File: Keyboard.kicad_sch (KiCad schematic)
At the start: 123 parts, among them SW1 MX_SW_solder, SW10 MX_SW_solder, SW11 MX_SW_solder, SW12 MX_SW_solder, SW13 MX_SW_solder, SW14 MX_SW_solder, SW15 MX_SW_solder, SW16 MX_SW_solder, SW17 MX_SW_solder, SW18 MX_SW_solder, SW19 MX_SW_solder, SW2 MX_SW_solder, SW20 MX_SW_solder, SW21 MX_SW_solder, SW22 MX_SW_solder, SW23 MX_SW_solder, SW24 MX_SW_solder, SW25 MX_SW_solder, SW26 MX_SW_solder, SW27 MX_SW_solder, SW28 MX_SW_solder, SW29 MX_SW_solder, SW3 MX_SW_solder, SW30 MX_SW_solder, SW31 MX_SW_solder, SW32 MX_SW_solder, SW33 MX_SW_solder, SW34 MX_SW_solder, SW35 MX_SW_solder, SW36 MX_SW_solder, SW37 MX_SW_solder, SW38 MX_SW_solder, SW39 MX_SW_solder, SW4 MX_SW_solder, SW40 MX_SW_solder, SW41 MX_SW_solder, SW42 MX_SW_solder, SW43 MX_SW_solder, SW44 MX_SW_solder, SW45 MX_SW_solder, SW46 MX_SW_solder, SW47 MX_SW_solder, SW48 MX_SW_solder, SW49 MX_SW_solder, SW5 MX_SW_solder, SW50 MX_SW_solder, SW51 MX_SW_solder, SW52 MX_SW_solder, SW53 MX_SW_solder, SW54 MX_SW_solder, SW55 MX_SW_solder, SW56 MX_SW_solder, SW57 MX_SW_solder, SW58 MX_SW_solder, SW59 MX_SW_solder, SW6 MX_SW_solder, SW60 MX_SW_solder, SW61 MX_SW_solder, SW7 MX_SW_solder, SW8 MX_SW_solder, SW9 MX_SW_solder, U1 Pico

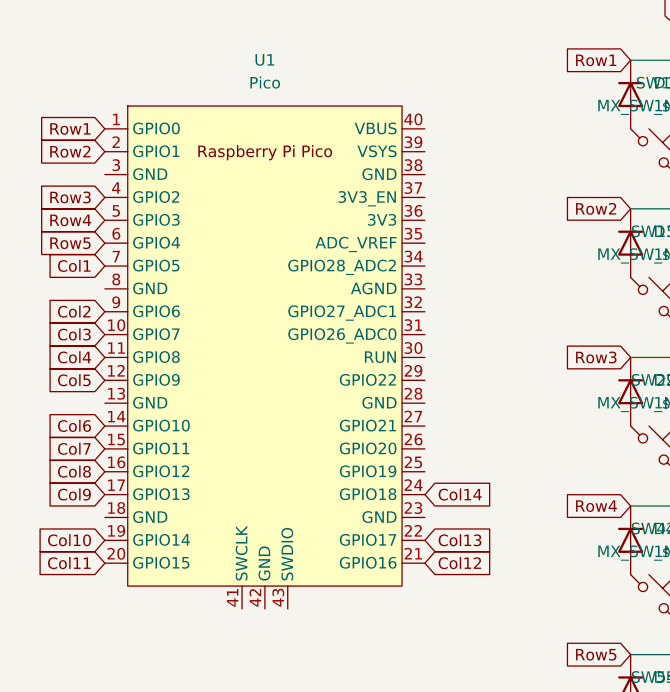
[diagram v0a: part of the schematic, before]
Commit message: Filled copper layer and added final touches
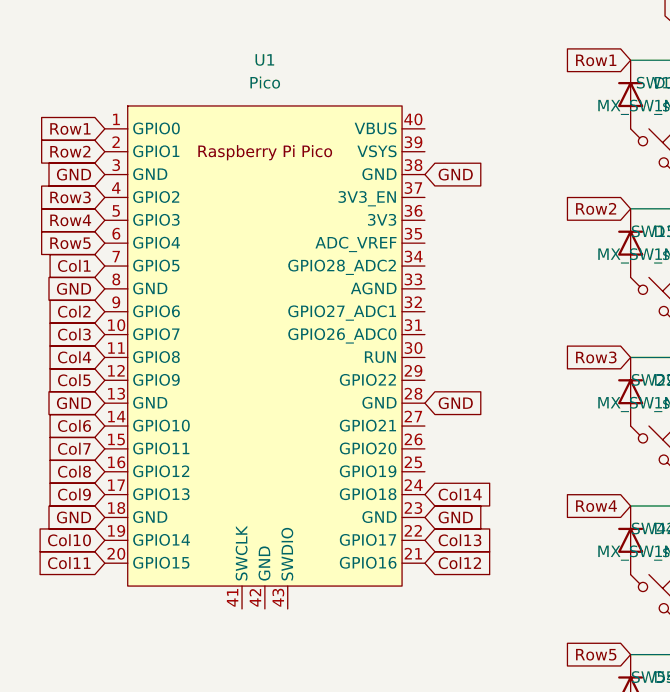
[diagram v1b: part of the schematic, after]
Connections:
- net GND: now reaches U1.13 (GND)
- net GND: now also U1.18 (GND), U1.23 (GND), U1.28 (GND), U1.3 (GND), U1.38 (GND), U1.8 (GND)
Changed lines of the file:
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@@
     (stroke (width 0) (type default) (color 0 0 0 0))
   )
+  (global_label "GND" (shape input) (at 66.04 74.93 0) (fields_autoplaced)
+    (effects (font (size 1.27 1.27)) (justify left))
+    (property "Intersheet References" "${INTERSHEET_REFS}" (id 0) (at 72.3236 74.8506 0)
+      (effects (font (size 1.27 1.27)) (justify left) hide)
+    )
+  )
   (global_label "Col1" (shape input) (at 93.98 20.32 90) (fields_autoplaced)
     (effects (font (size 1.27 1.27)) (justify left))
@@
     )
   )
+  (global_label "GND" (shape input) (at 30.48 36.83 180) (fields_autoplaced)
+    (effects (font (size 1.27 1.27)) (justify right))
+    (property "Intersheet References" "${INTERSHEET_REFS}" (id 0) (at 24.1964 36.9094 0)
+      (effects (font (size 1.27 1.27)) (justify right) hide)
+    )
+  )
   (global_label "Row4" (shape input) (at 88.9 73.66 180) (fields_autoplaced)
     (effects (font (size 1.27 1.27)) (justify right))
@@
     )
   )
+  (global_label "GND" (shape input) (at 66.04 62.23 0) (fields_autoplaced)
+    (effects (font (size 1.27 1.27)) (justify left))
+    (property "Intersheet References" "${INTERSHEET_REFS}" (id 0) (at 72.3236 62.1506 0)
+      (effects (font (size 1.27 1.27)) (justify left) hide)
+    )
+  )
   (global_label "Col14" (shape input) (at 66.04 72.39 0) (fields_autoplaced)
     (effects (font (size 1.27 1.27)) (justify left))
@@
     )
   )
+  (global_label "GND" (shape input) (at 30.48 62.23 180) (fields_autoplaced)
+    (effects (font (size 1.27 1.27)) (justify right))
+    (property "Intersheet References" "${INTERSHEET_REFS}" (id 0) (at 24.1964 62.3094 0)
+      (effects (font (size 1.27 1.27)) (justify right) hide)
+    )
+  )
   (global_label "Col3" (shape input) (at 30.48 54.61 180) (fields_autoplaced)
     (effects (font (size 1.27 1.27)) (justify right))
@@
     )
   )
+  (global_label "GND" (shape input) (at 30.48 74.93 180) (fields_autoplaced)
+    (effects (font (size 1.27 1.27)) (justify right))
+    (property "Intersheet References" "${INTERSHEET_REFS}" (id 0) (at 24.1964 75.0094 0)
+      (effects (font (size 1.27 1.27)) (justify right) hide)
+    )
+  )
   (global_label "Col5" (shape input) (at 129.54 20.32 90) (fields_autoplaced)
     (effects (font (size 1.27 1.27)) (justify left))
@@
     )
   )
+  (global_label "GND" (shape input) (at 66.04 36.83 0) (fields_autoplaced)
+    (effects (font (size 1.27 1.27)) (justify left))
+    (property "Intersheet References" "${INTERSHEET_REFS}" (id 0) (at 72.3236 36.7506 0)
+      (effects (font (size 1.27 1.27)) (justify left) hide)
+    )
+  )
   (global_label "Col9" (shape input) (at 30.48 72.39 180) (fields_autoplaced)
     (effects (font (size 1.27 1.27)) (justify right))
@@
       (effects (font (size 1.27 1.27)) (justify right) hide)
     )
+  )
+  (global_label "GND" (shape input) (at 30.48 49.53 180) (fields_autoplaced)
+    (effects (font (size 1.27 1.27)) (justify right))
+    (property "Intersheet References" "${INTERSHEET_REFS}" (id 0) (at 24.1964 49.6094 0)
+      (effects (font (size 1.27 1.27)) (justify right) hide)
+    )

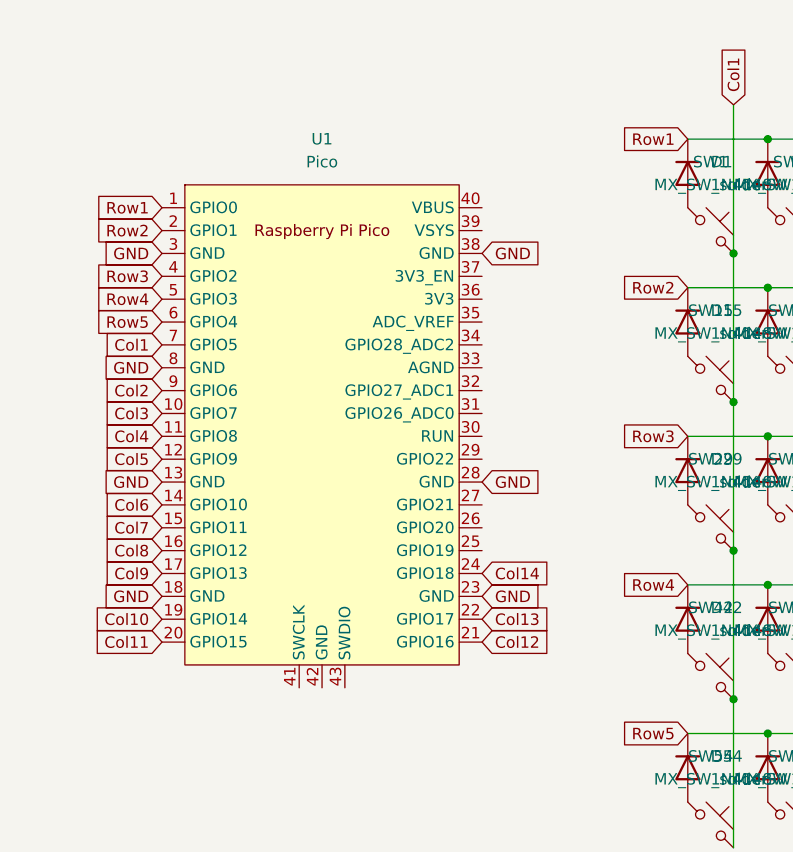
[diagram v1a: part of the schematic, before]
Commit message: Added Pcb Art
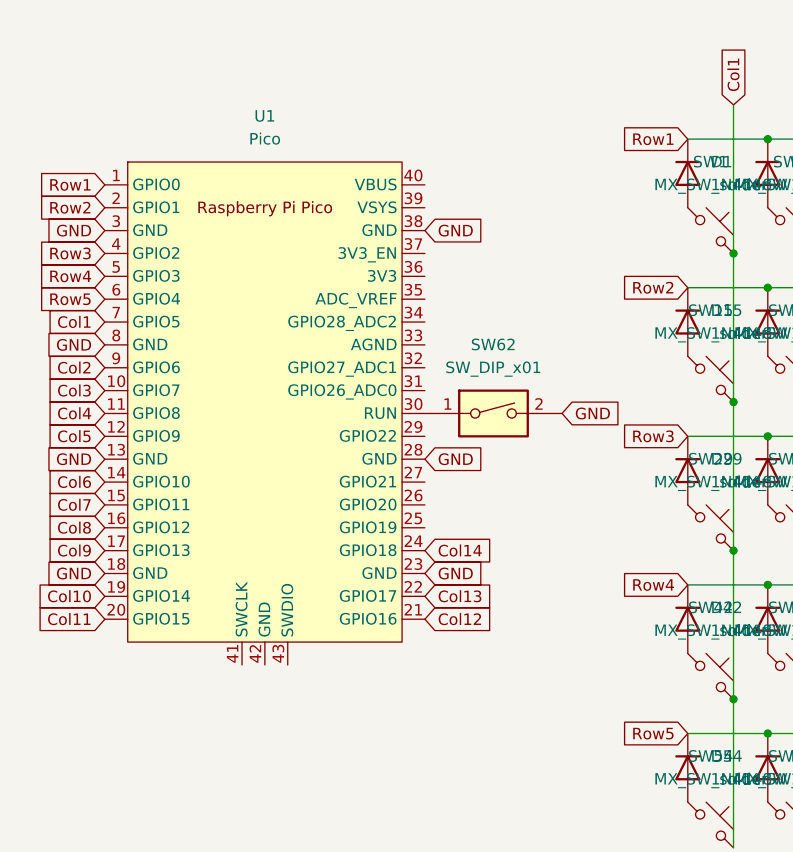
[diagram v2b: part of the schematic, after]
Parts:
- added SW62: SW_DIP_x01, Button_Switch_THT:SW_PUSH_6mm, symbol Switch:SW_DIP_x01
- D1, D10, D11, D12, D13, D14, D15, D16, D17, D18, D19, D2, D20, D21, D22, D23, D24, D25, D26, D27, D28, D29, D3, D30, D31, D32, D33, D34, D35, D36, D37, D38, D39, D4, D40, D41, D42, D43, D44, D45, D46, D47, D48, D49, D5, D50, D51, D52, D53, D54, D55, D56, D57, D58, D59, D6, D60, D61, D7, D8, D9: LCSC (none) -> C81598
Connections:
- net GND: now also SW62.2
- net at U1.30 (RUN): now also SW62.1
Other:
- title: (none) -> 60% keyboard
- moved on the sheet: U1
